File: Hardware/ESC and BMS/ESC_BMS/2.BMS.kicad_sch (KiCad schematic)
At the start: 38 parts, among them J301 SW IN, J302 SW OUT, Q301 SQJQ131EL, Q303 FDV304P, Q304 PMV20XNEA, Q305 SQJQ131EL, Q306 SQJQ131EL, U301 BQ2057W, U302 BQ2969

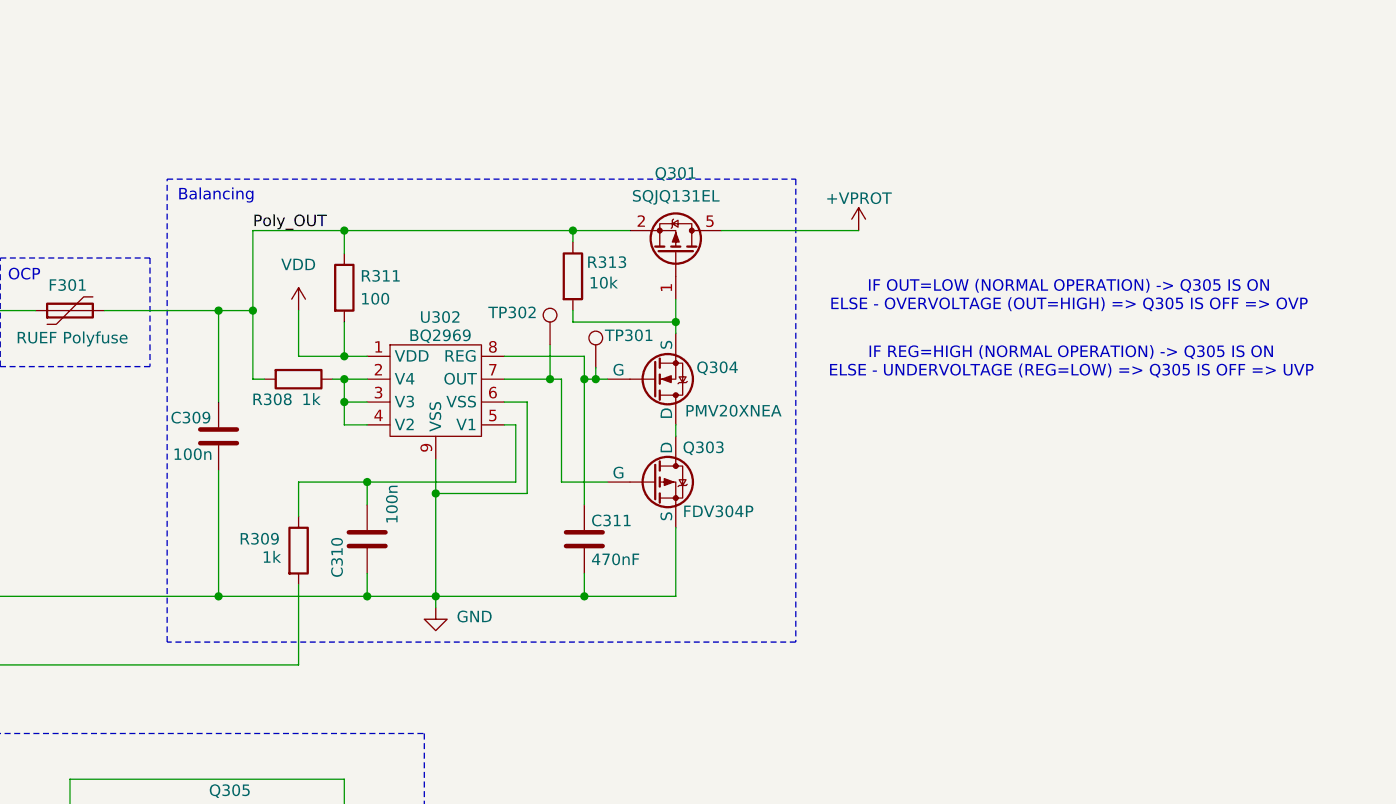
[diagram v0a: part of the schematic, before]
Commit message: Minor adjustments to BMS schematic - beautifying
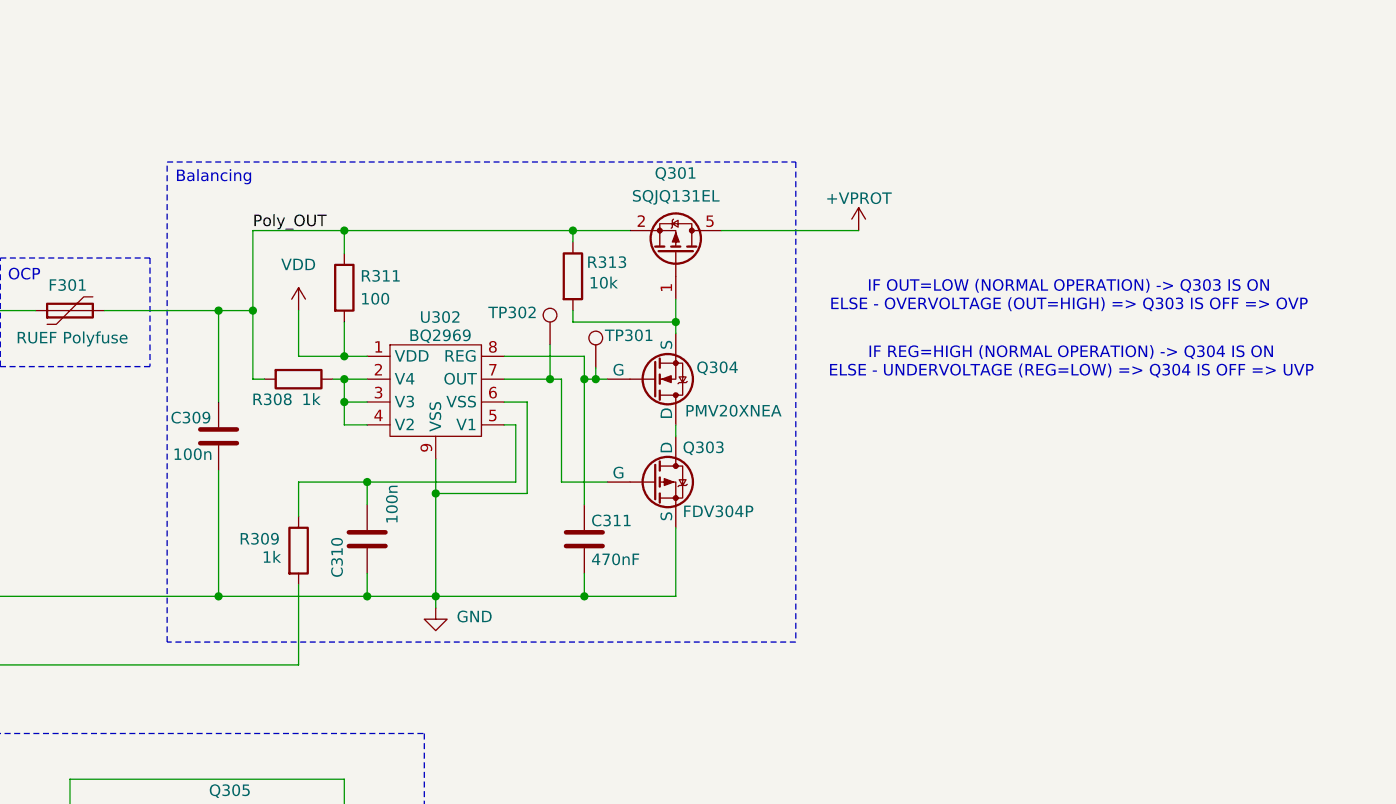
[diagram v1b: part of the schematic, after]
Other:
- note added: "IF OUT=LOW (NORMAL OPERATION) -> Q303 IS ON ELSE - OVERVOLTAGE (OUT=HIGH) => Q303 IS OFF => OVP"
- note added: "IF REG=HIGH (NORMAL OPERATION) -> Q304 IS ON ELSE - UNDERVOLTAGE (REG=LOW) => Q304 IS OFF => UVP"
- note removed: "IF OUT=LOW (NORMAL OPERATION) -> Q305 IS ON ELSE - OVERVOLTAGE (OUT=HIGH) => Q305 IS OFF => OVP"
- note removed: "IF REG=HIGH (NORMAL OPERATION) -> Q305 IS ON ELSE - UNDERVOLTAGE (REG=LOW) => Q305 IS OFF => UVP"
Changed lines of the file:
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@@
 	)
 	(rectangle
-		(start 196.215 80.645)
+		(start 196.215 78.74)
 		(end 266.065 132.08)
 		(stroke
@@
 		)
 	)
-	(text "IF OUT=LOW (NORMAL OPERATION) -> Q305 IS ON\nELSE - OVERVOLTAGE (OUT=HIGH) => Q305 IS OFF => OVP"
+	(text "IF OUT=LOW (NORMAL OPERATION) -> Q303 IS ON\nELSE - OVERVOLTAGE (OUT=HIGH) => Q303 IS OFF => OVP"
 		(exclude_from_sim no)
 		(at 296.418 93.726 0)
@@
 		)
 	)
-	(text "IF REG=HIGH (NORMAL OPERATION) -> Q305 IS ON\nELSE - UNDERVOLTAGE (REG=LOW) => Q305 IS OFF => UVP"
+	(text "IF REG=HIGH (NORMAL OPERATION) -> Q304 IS ON\nELSE - UNDERVOLTAGE (REG=LOW) => Q304 IS OFF => UVP"
 		(exclude_from_sim no)
 		(at 296.672 101.092 0)
@@
 	(text "Balancing"
 		(exclude_from_sim no)
-		(at 201.676 82.55 0)
+		(at 201.422 80.518 0)
 		(effects
 			(font
